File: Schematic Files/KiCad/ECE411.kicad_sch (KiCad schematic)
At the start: 9 parts, among them J1-ToPump1 Conn_01x02_Female, J2-ToMoistSense1 Conn_01x02_Female, Q1 2N7002

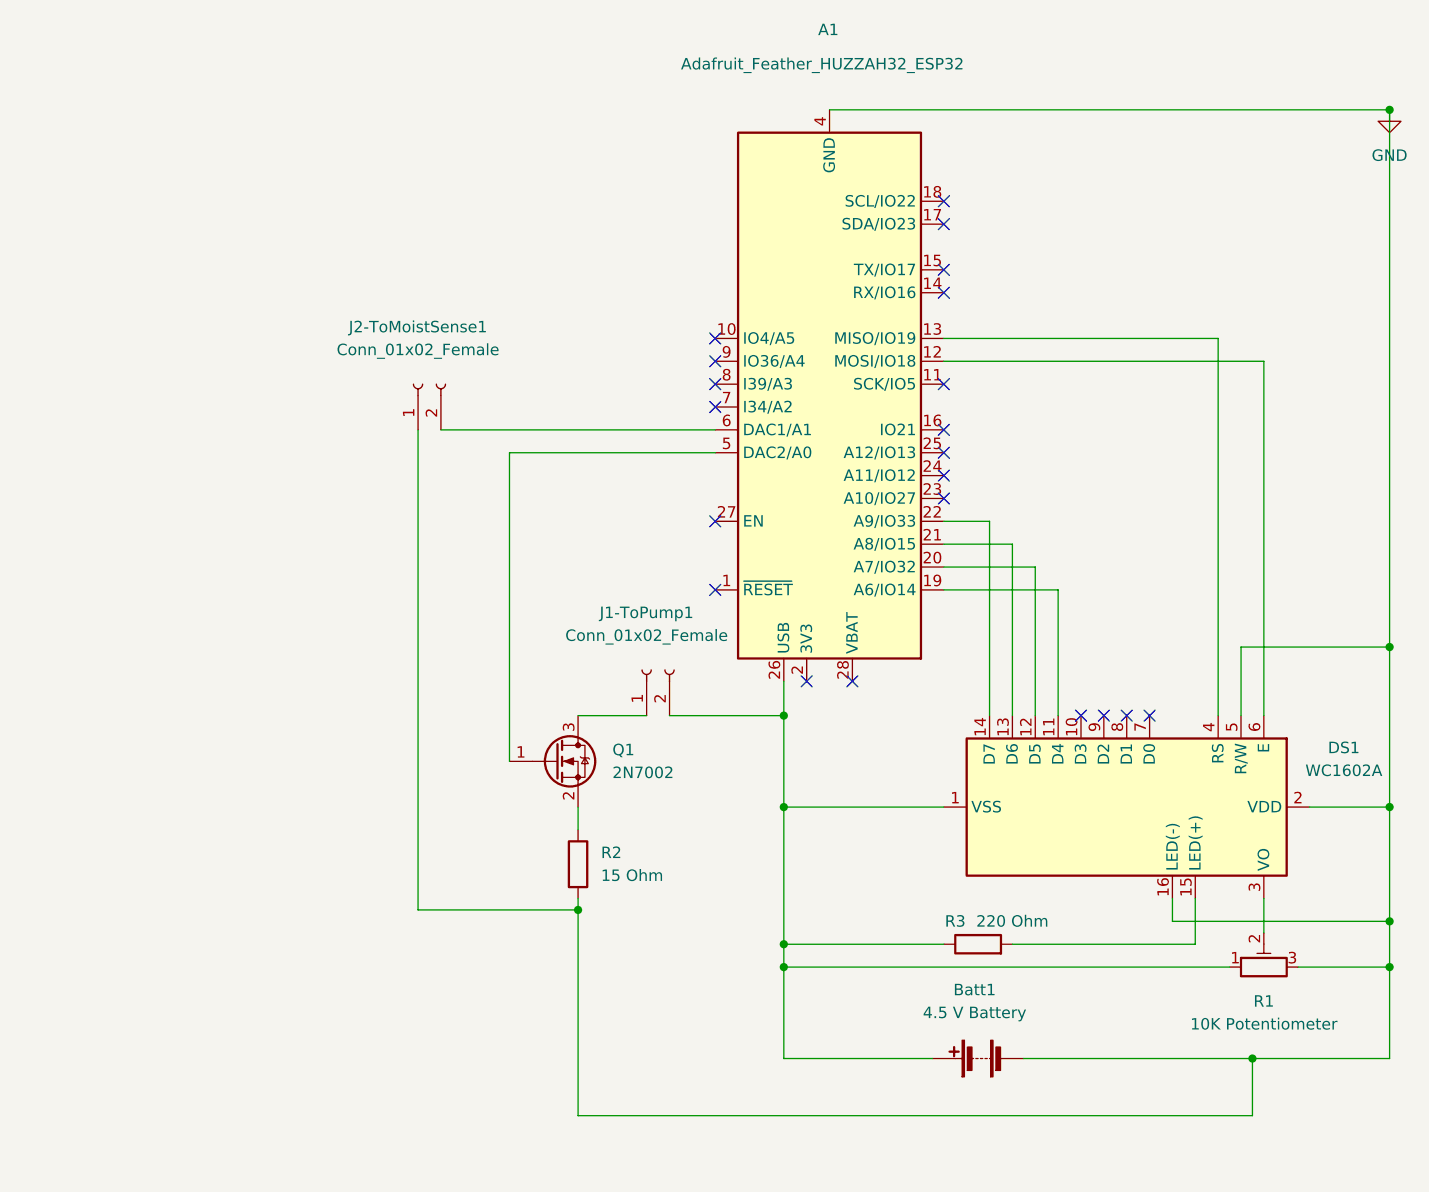
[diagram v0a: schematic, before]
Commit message: Add files via upload
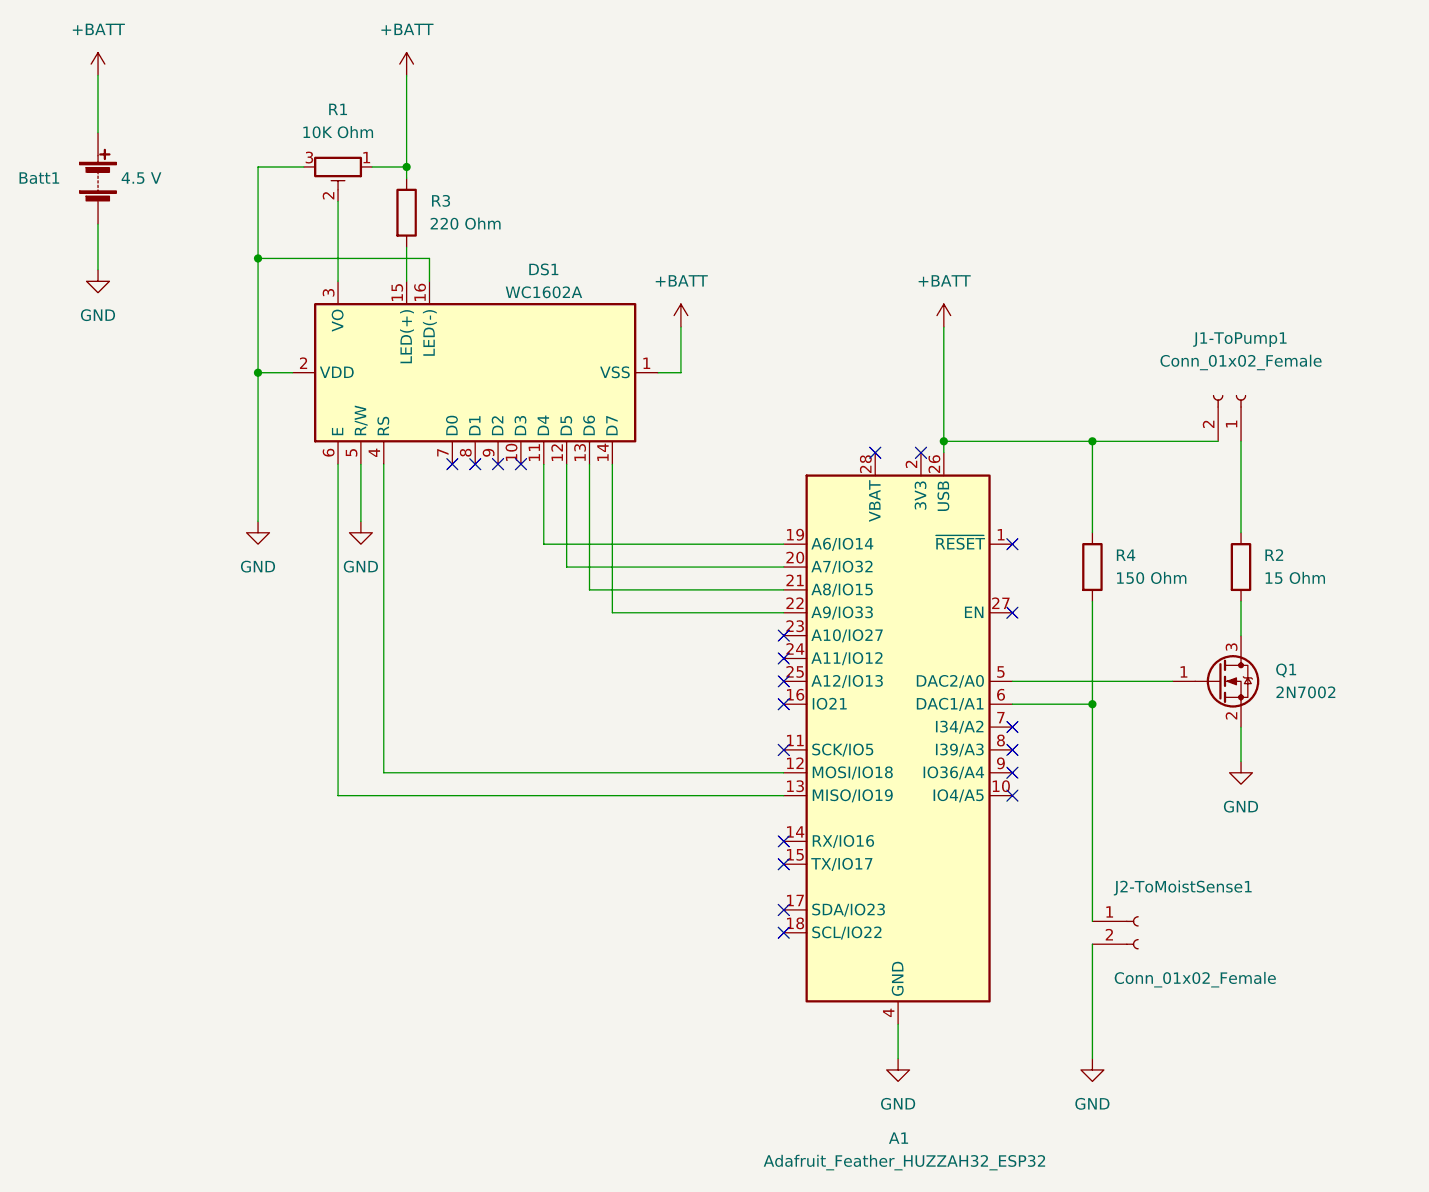
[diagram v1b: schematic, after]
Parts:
- added R4: 150 Ohm, Resistor_SMD:R_1206_3216Metric, symbol Device:R
- Batt1: value 4.5 V Battery -> 4.5 V
- R1: value 10K Potentiometer -> 10K Ohm
- R2, R3: footprint Resistor_SMD:R_0402_1005Metric -> Resistor_SMD:R_1206_3216Metric
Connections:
- net GND: now also J2-ToMoistSense1.2 (Pin_2), Q1.2 (S); no longer J2-ToMoistSense1.1 (Pin_1), R2.2
- net at J1-ToPump1.1 (Pin_1): now also R2.1; no longer Q1.3 (D)
- net +BATT: now reaches A1.26 (USB), Batt1.1 (+), DS1.1 (VSS), J1-ToPump1.2 (Pin_2), R1.1, R3.1
- net +BATT: now also R4.1
- net at A1.12 (MOSI/IO18): now also DS1.4 (RS); no longer DS1.6 (E)
- net at A1.13 (MISO/IO19): now also DS1.6 (E); no longer DS1.4 (RS)
- net at A1.6 (DAC1/A1): now also J2-ToMoistSense1.1 (Pin_1), R4.2; no longer J2-ToMoistSense1.2 (Pin_2)
- new net: Q1.3 (D), R2.2
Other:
- company: (none) -> Frantic Four
- title: (none) -> Thirsty Plants PCB
- moved on the sheet: A1, Batt1, DS1, J1-ToPump1, J2-ToMoistSense1, Q1, R1, R2, R3
